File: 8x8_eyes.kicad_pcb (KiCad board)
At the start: 2 copper layers, 71.1 x 63.5 mm, 13 parts, among them J1 Conn_01x05_Female, U1 74HC595, U2 74HC595

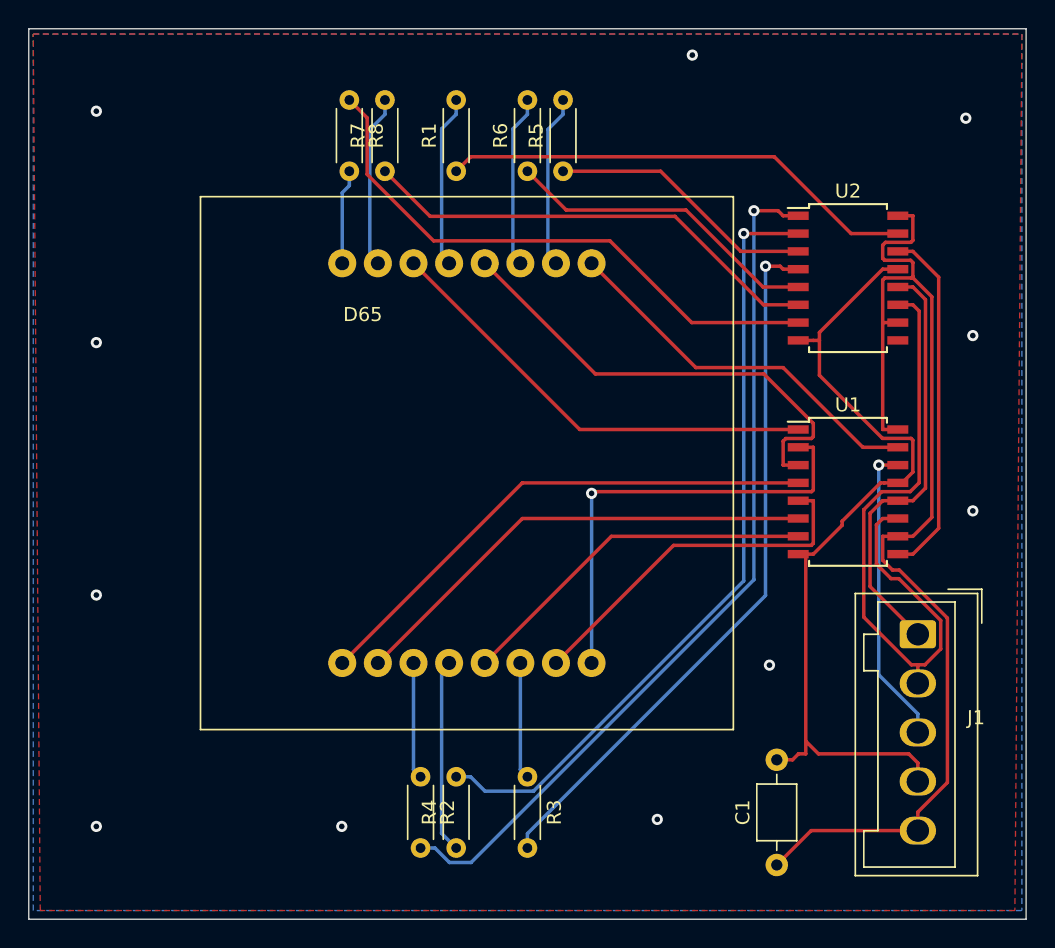
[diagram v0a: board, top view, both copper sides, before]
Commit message: fix
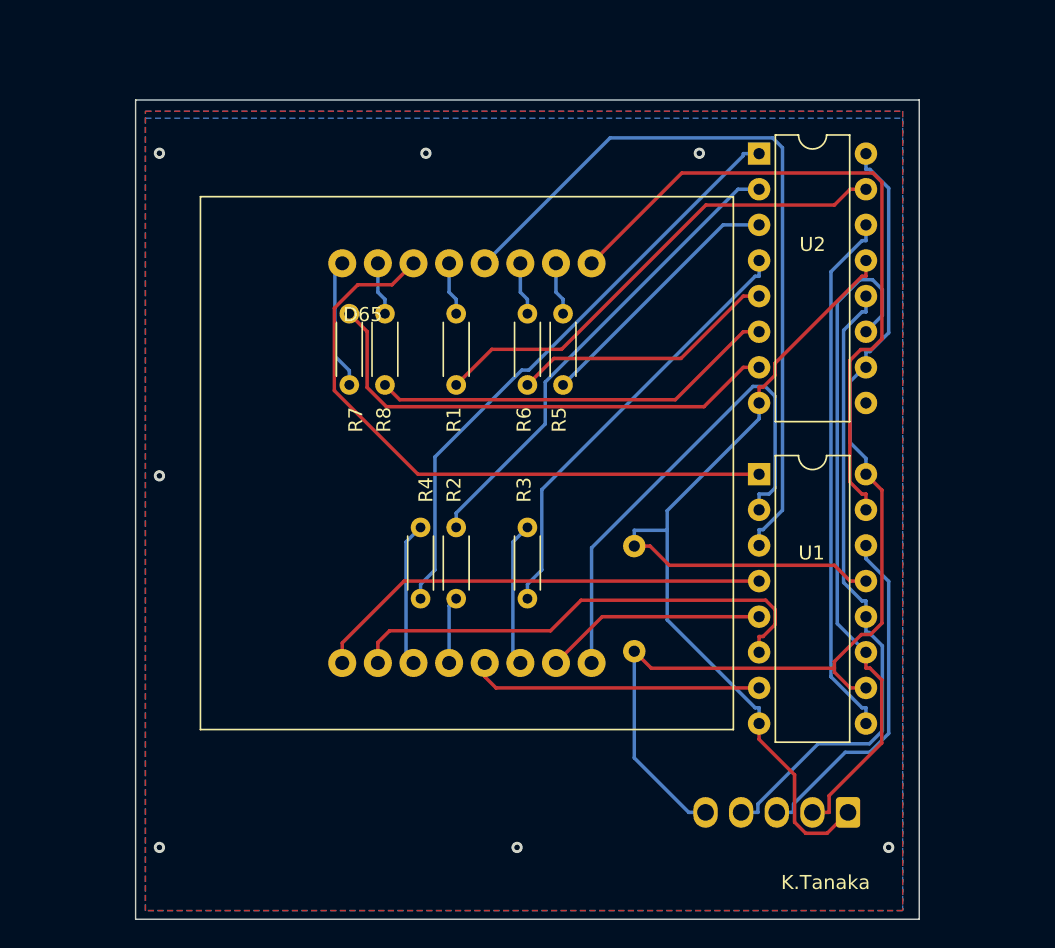
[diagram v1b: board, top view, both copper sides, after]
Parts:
- C1: moved to B.Cu
- J1: footprint Connector_Wago:Wago_734-135_1x05_P3.50mm_Vertical -> Connector_Molex:Molex_KK-254_AE-6410-05A_1x05_P2.54mm_Vertical; moved to B.Cu
- U1, U2: footprint Package_SO:SOIC-16W_5.3x10.2mm_P1.27mm -> Package_DIP:DIP-16_W7.62mm
- moved C1 18.3 mm to (149.9, 115.5)
- moved R2 17.8 mm to (134.6, 106.7)
- moved R3 17.8 mm to (142.2, 106.7)
- moved R4 17.8 mm to (137.2, 111.8)
- moved R1 15.2 mm to (137.2, 96.5)
- moved R5 15.2 mm to (144.8, 96.5)
- moved R6 15.2 mm to (142.2, 96.5)
- moved R7 15.2 mm to (132.1, 96.5)
- moved R8 15.2 mm to (129.5, 91.4)
- moved J1 13.6 mm to (165.1, 127.0), turned to 180 degrees
- moved U2 10.9 mm to (158.8, 80.0)
- moved U1 6.46 mm to (158.8, 102.9)
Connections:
- J1 pad 1: CLR -> GND
- J1 pad 4: GND -> CLR
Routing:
- net Pin 4: track 55.8 -> 33.9 mm, vias 1 -> 0
- net Pin 9: track 27.3 -> 49.0 mm
- net Pin 12: track 34.2 -> 54.4 mm
- net Pin 6: track 50.9 -> 31.1 mm, vias 1 -> 0
- net Pin 3: track 62.2 -> 42.7 mm, vias 1 -> 0
- net GND: track 60.1 -> 76.0 mm, vias 11 -> 7
- net CLR: track 30.5 -> 46.1 mm
- net Pin 14: track 32.3 -> 45.6 mm
- net CASCADE: track 25.3 -> 38.0 mm
- net Pin 7: track 26.0 -> 15.9 mm
- net Net-(D65-Pad4): track 13.8 -> 4.79 mm
- net Net-(D65-Pad10): track 12.3 -> 3.80 mm
- net Net-(D65-Pad15): track 12.3 -> 3.80 mm
- net Net-(D65-Pad11): track 12.3 -> 3.80 mm
- net Net-(D65-Pad13): track 12.3 -> 3.80 mm
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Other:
- board size 71.1 x 63.5 mm -> 55.9 x 58.4 mm
- board text added: "1"
- board text added: "2"
- board text added: "3"
- board text added: "4"
- board text added: "5"
- board text added: "CLK"
- board text added: "CLR"
- board text added: "GND"
- board text added: "K.Tanaka"
- board text added: "SER"
- board text added: "VCC"
